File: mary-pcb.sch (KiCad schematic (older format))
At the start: 69 parts, among them SW1 SW_Push, SW2 Rotary_Encoder_Switch, U1 ATmega32U4-AU, Y1 16MHz

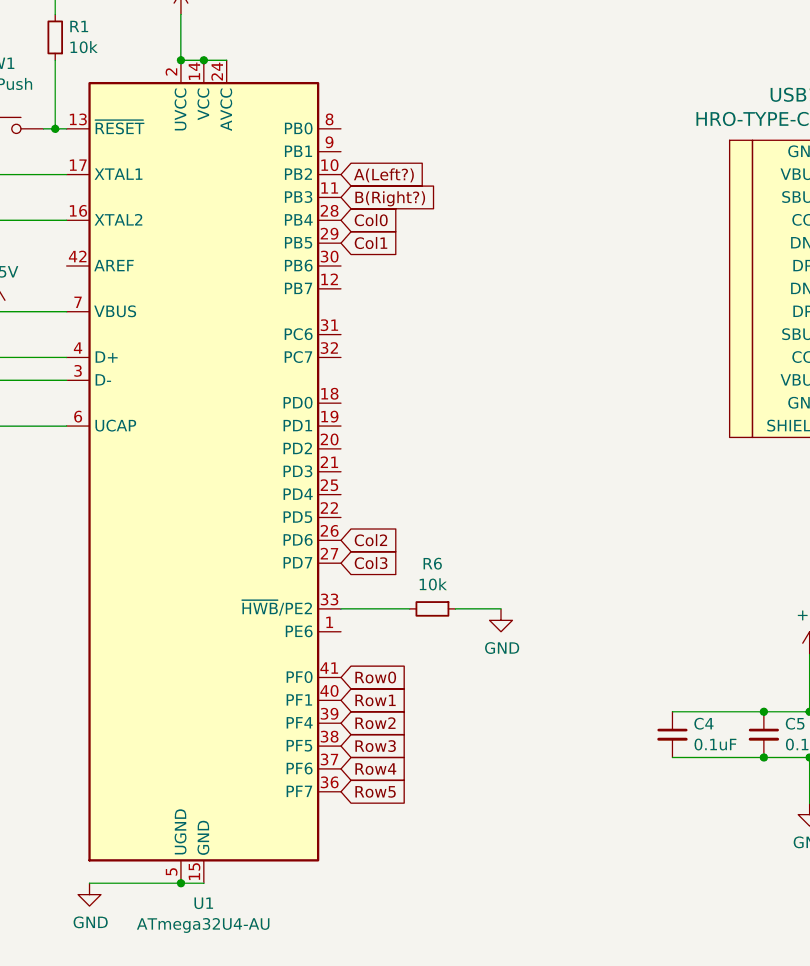
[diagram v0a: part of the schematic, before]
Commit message: complete routing, upload renders
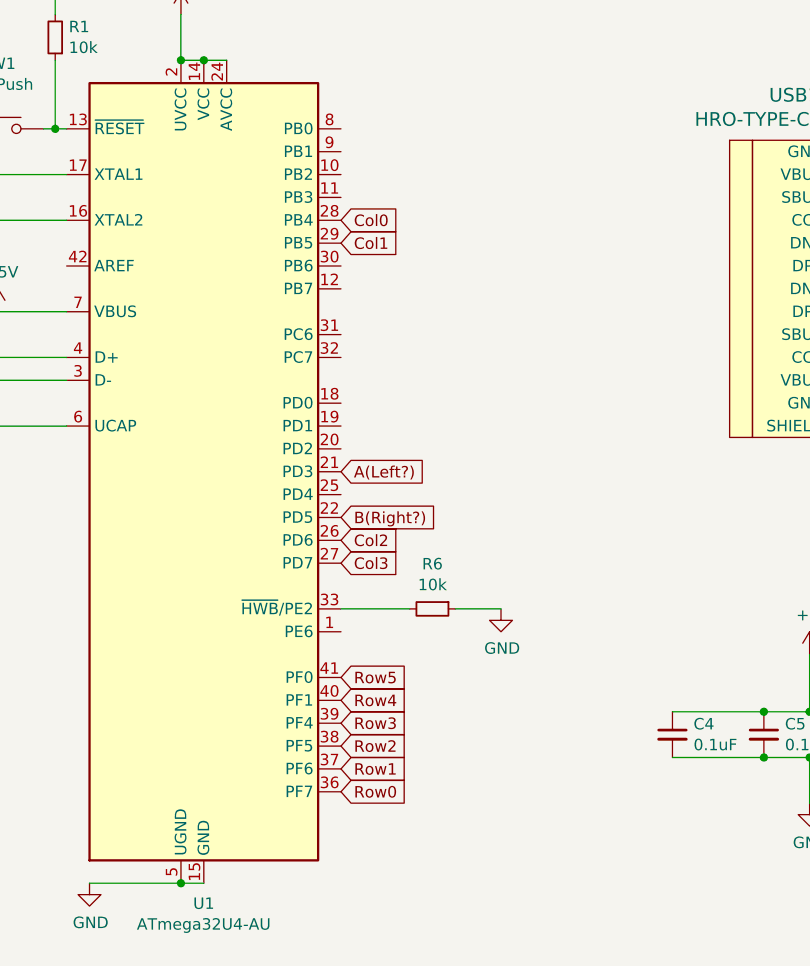
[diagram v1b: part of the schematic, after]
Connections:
- net A(Left?): now also U1.21 (PD3); no longer U1.10 (PB2)
- net B(Right?): now also U1.22 (PD5); no longer U1.11 (PB3)
- net Row0: now also U1.36 (PF7); no longer U1.41 (PF0)
- net Row1: now also U1.37 (PF6); no longer U1.40 (PF1)
- net Row2: now also U1.38 (PF5); no longer U1.39 (PF4)
- net Row3: now also U1.39 (PF4); no longer U1.38 (PF5)
- net Row4: now also U1.40 (PF1); no longer U1.37 (PF6)
- net Row5: now also U1.41 (PF0); no longer U1.36 (PF7)
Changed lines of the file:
@@
 	10500 2250 10500 2450
 Connection ~ 10500 2450
-Text GLabel 3450 3850 2    50   Input ~ 0
-Row0
-Text GLabel 3450 3950 2    50   Input ~ 0
-Row1
-Text GLabel 3450 4050 2    50   Input ~ 0
-Row2
-Text GLabel 3450 4150 2    50   Input ~ 0
-Row3
-Text GLabel 3450 4250 2    50   Input ~ 0
-Row4
-Text GLabel 3450 4350 2    50   Input ~ 0
-Row5
-Text GLabel 3450 1850 2    50   Input ~ 0
-Col0
-Text GLabel 3450 1950 2    50   Input ~ 0
-Col1
-Text GLabel 3450 3250 2    50   Input ~ 0
-Col2
-Text GLabel 3450 3350 2    50   Input ~ 0
-Col3
 $Comp
 L Device:D_Small D4
@@
 	10350 2050 10350 1950
 Connection ~ 10350 1950
-Text GLabel 3450 1650 2    50   Input ~ 0
+Text GLabel 3450 3850 2    50   Input ~ 0
+Row5
+Text GLabel 3450 3950 2    50   Input ~ 0
+Row4
+Text GLabel 3450 4050 2    50   Input ~ 0
+Row3
+Text GLabel 3450 4150 2    50   Input ~ 0
+Row2
+Text GLabel 3450 4250 2    50   Input ~ 0
+Row1
+Text GLabel 3450 4350 2    50   Input ~ 0
+Row0
+Text GLabel 3450 1850 2    50   Input ~ 0
+Col0
+Text GLabel 3450 3350 2    50   Input ~ 0
+Col3
+Text GLabel 3450 3250 2    50   Input ~ 0
+Col2
+Text GLabel 3450 1950 2    50   Input ~ 0
+Col1
+Text GLabel 3450 2950 2    50   Input ~ 0
 A(Left?)
-Text GLabel 3450 1750 2    50   Input ~ 0
+Text GLabel 3450 3150 2    50   Input ~ 0
 B(Right?)
 $EndSCHEMATC
